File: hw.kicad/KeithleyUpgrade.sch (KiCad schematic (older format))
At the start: 75 parts, among them J1 DEBUG_PORT, J14 DISPLAY_BOARD, K1 TRIGGER, P1 TC2030-MCP, P18 CONN_8, P8 TP1, P9 TP1, Q1 BC850, U1 24AA256, U2 FT230x, U3 PIC32MX350F128L, U4 MIC2981, U5 MIC2981, U6 LM2936, U7 TMP275, U8 4050, X1 CRYSTAL_SMD_4POL

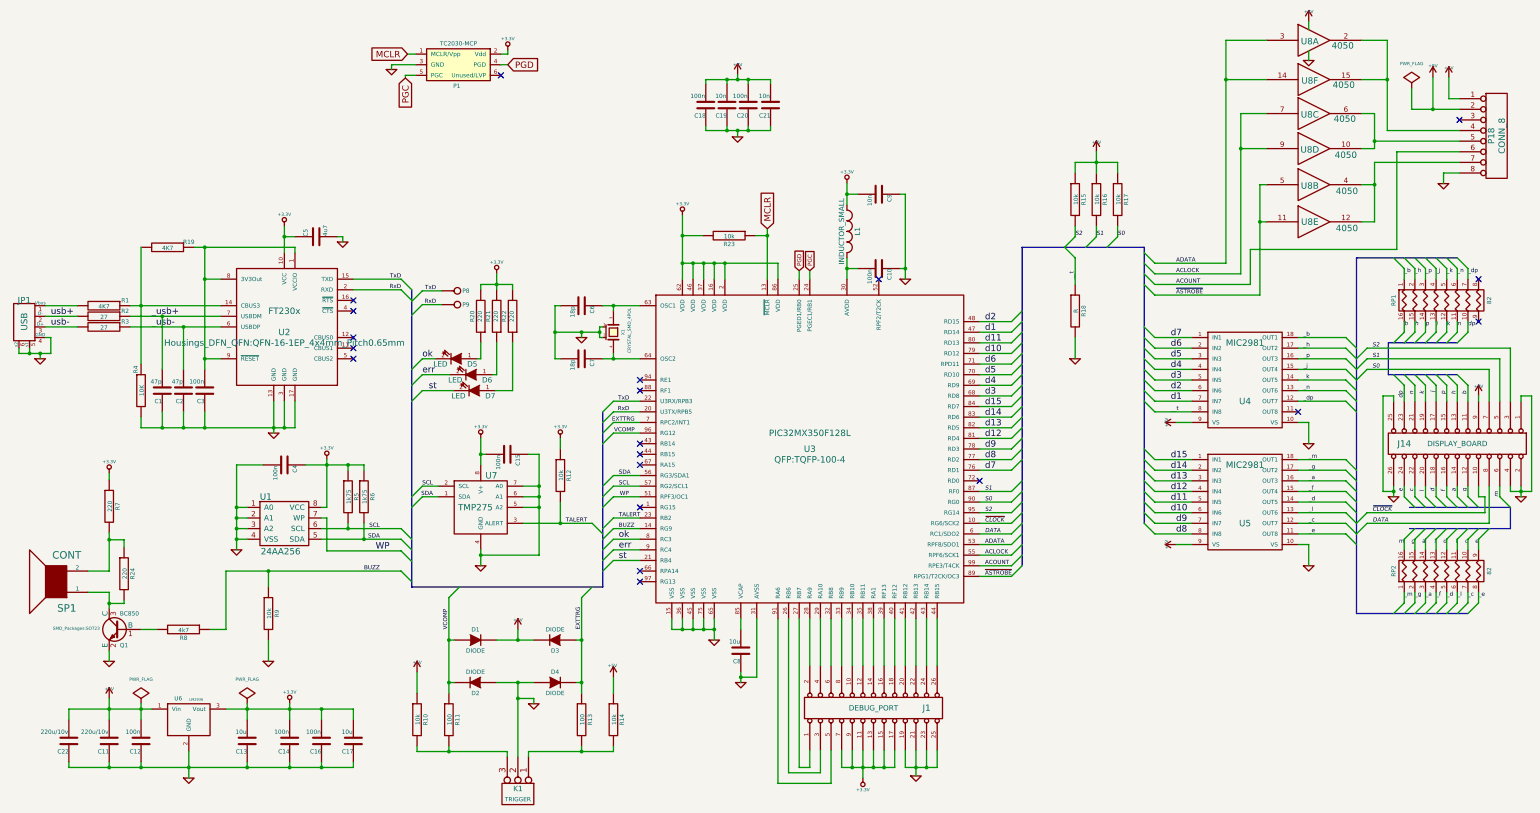
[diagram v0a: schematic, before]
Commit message: addedd documentation@
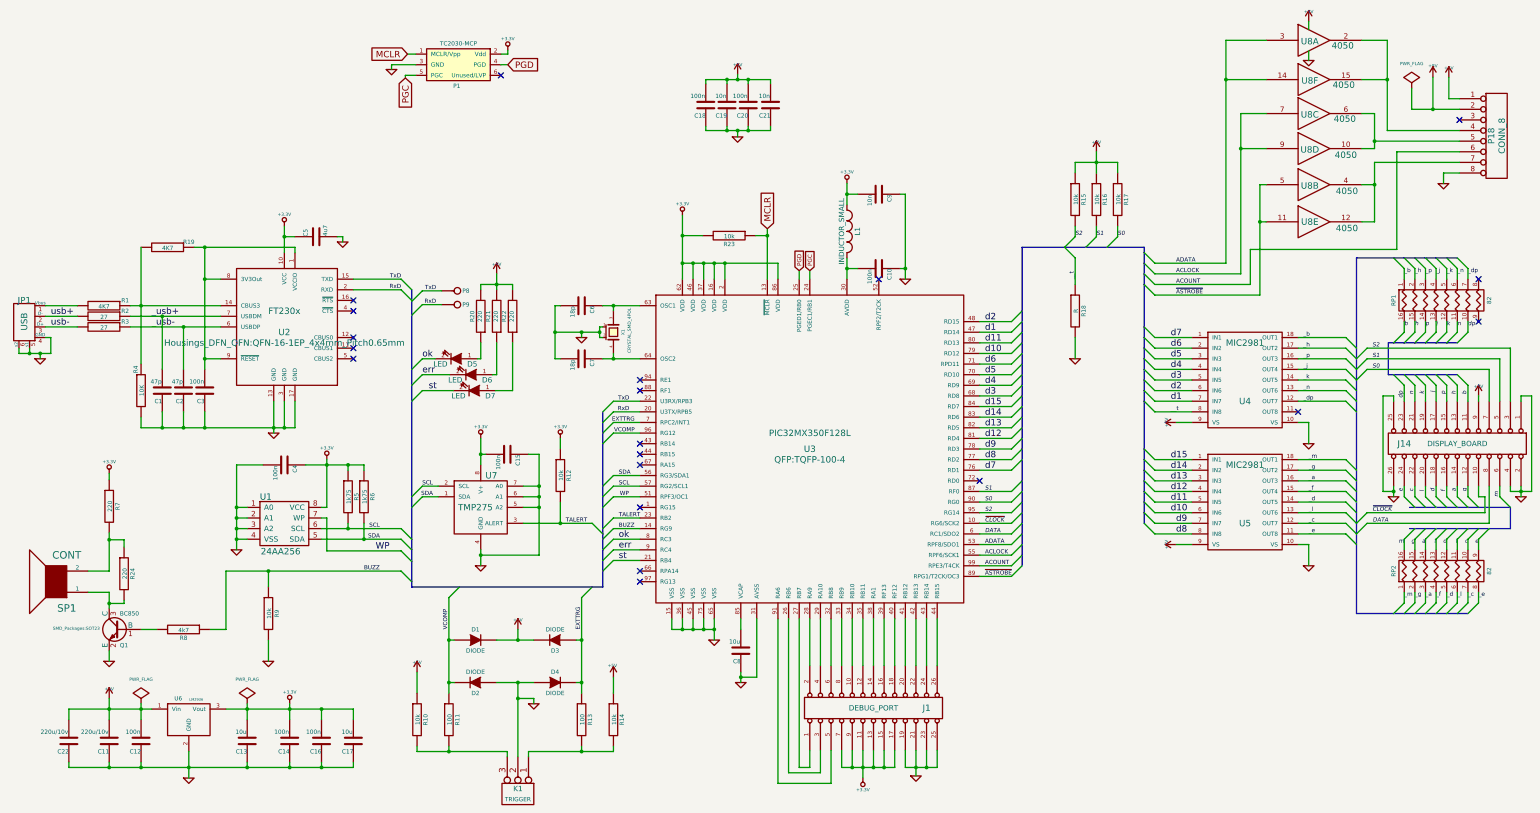
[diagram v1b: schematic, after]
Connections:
- net +3.3V: no longer R20.2, R21.2, R22.2
- net +5V: now also R20.2, R21.2, R22.2
- net at U3.43 (RB14): now also J1.24 (P20)
- net at U3.44 (RB15): now also J1.26 (P22)

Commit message: update documentation
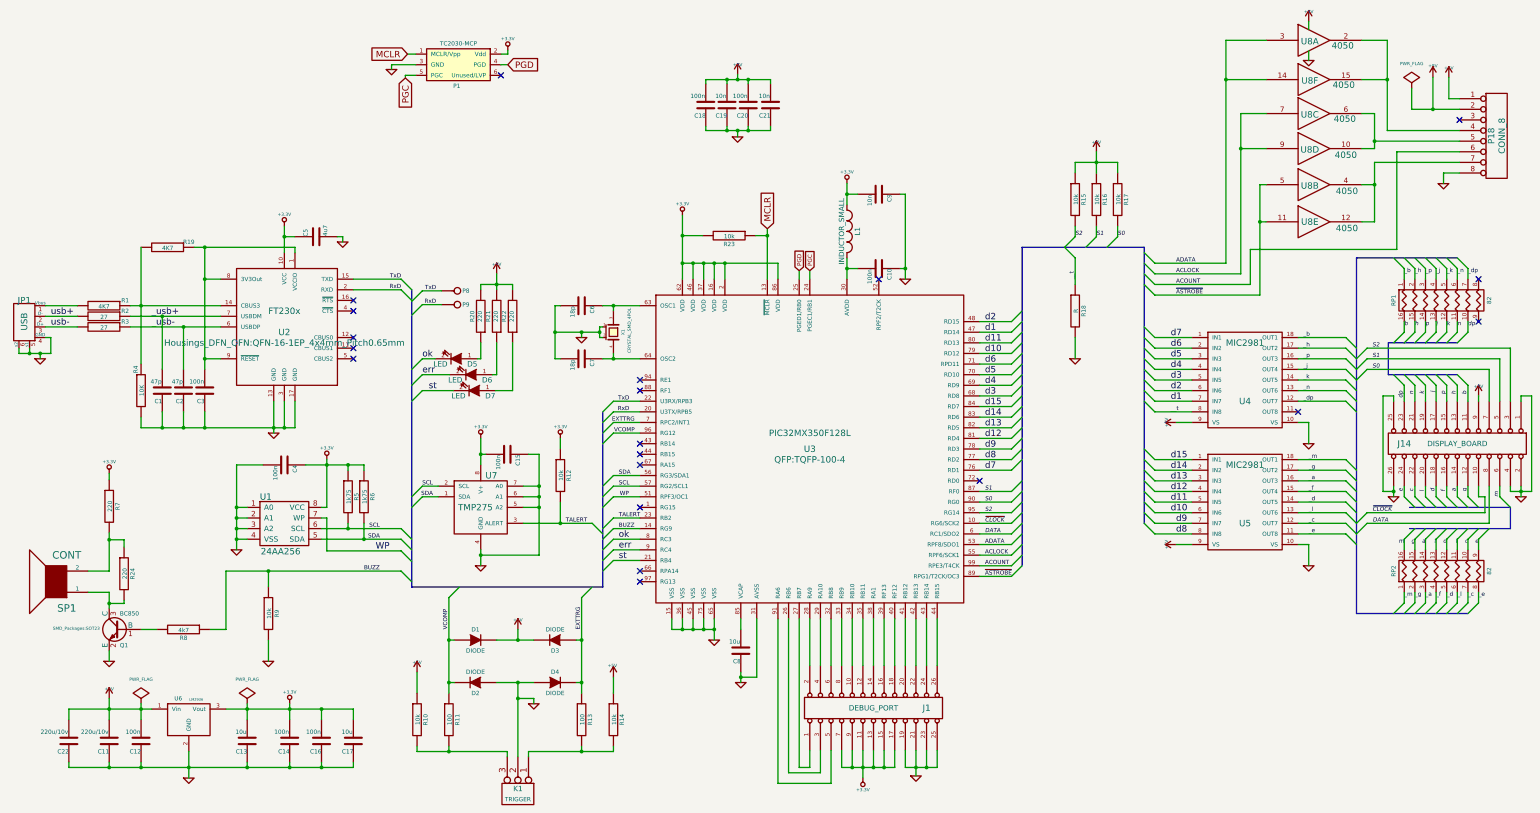
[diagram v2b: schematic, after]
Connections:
- net at U3.43 (RB14): now also J1.24 (P20)
- net at U3.44 (RB15): now also J1.26 (P22)
